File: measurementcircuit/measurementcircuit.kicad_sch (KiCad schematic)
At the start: 17 parts, among them J1 Conn_01x05_Socket, J2 Conn_01x05_Socket

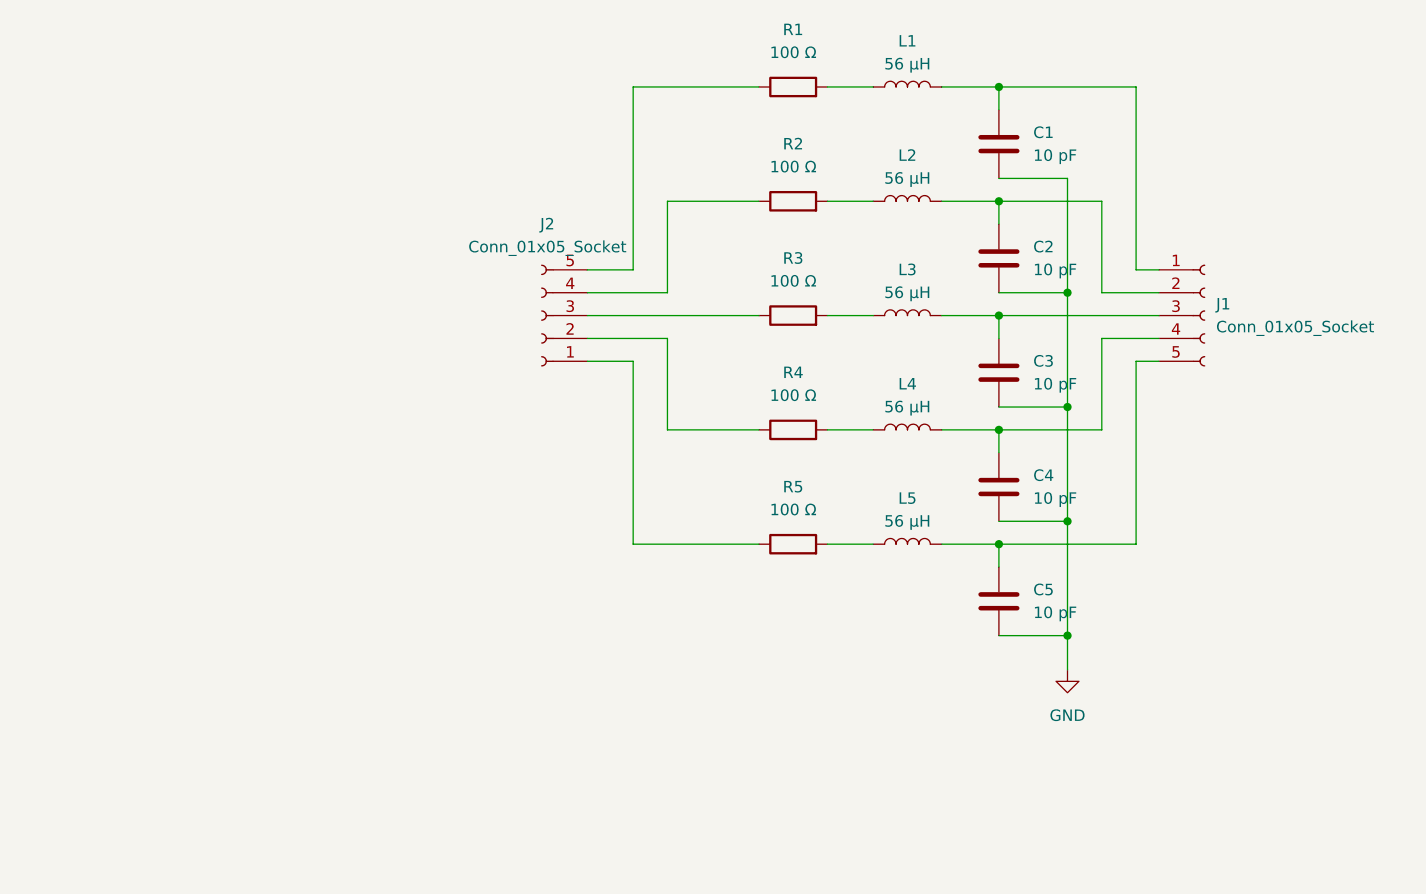
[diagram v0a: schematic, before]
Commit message: Only missing POT
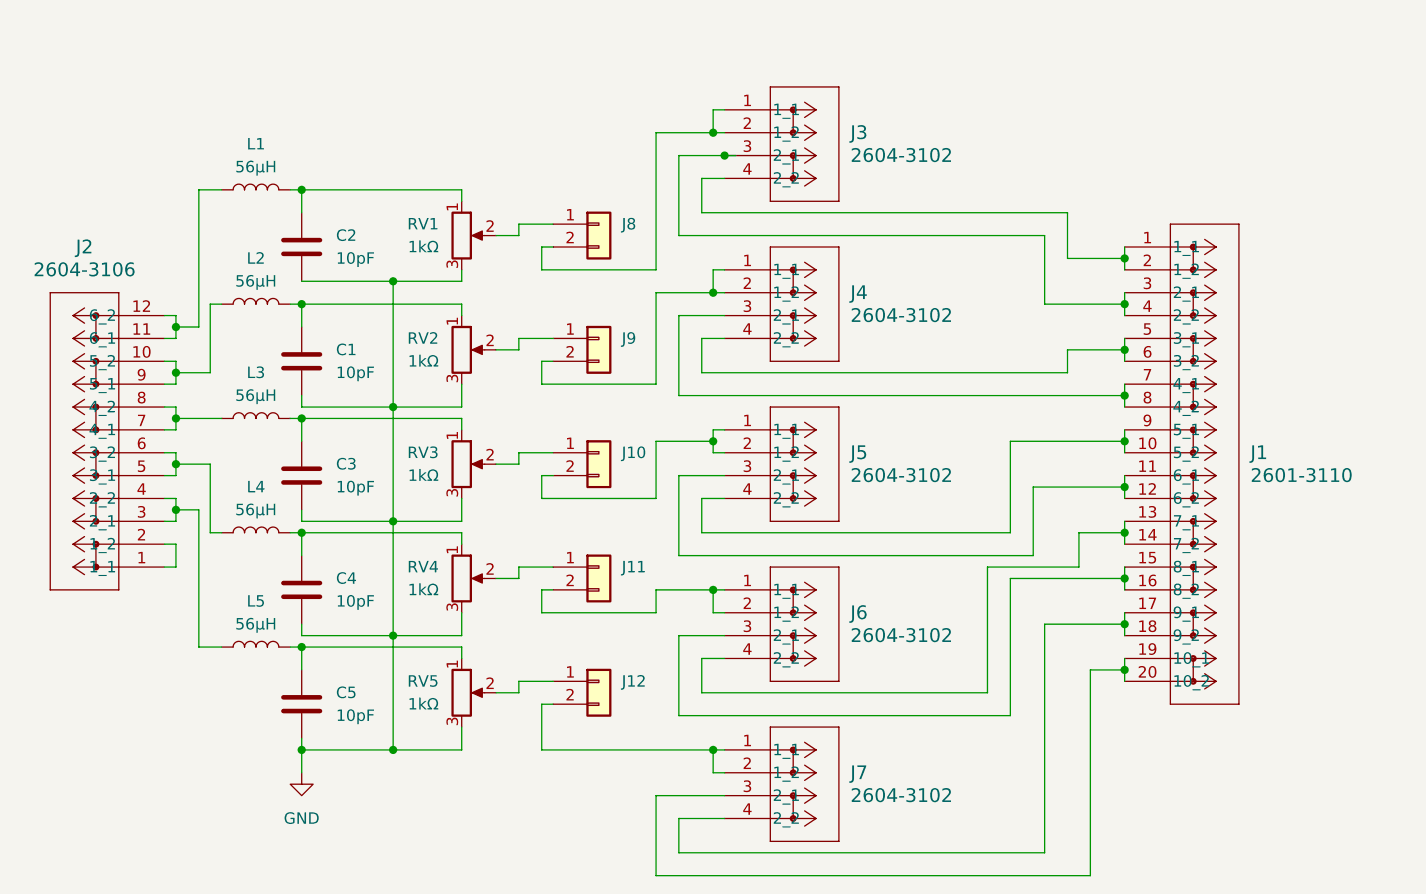
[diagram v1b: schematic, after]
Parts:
- removed J1, J2: Conn_01x05_Socket, Connector_Pin:Pin_D1.3mm_L10.0mm_W3.5mm_Flat, symbol Connector:Conn_01x05_Socket
- removed R1, R2, R3, R4, R5: 100 Ω, Resistor_THT:R_Axial_DIN0204_L3.6mm_D1.6mm_P5.08mm_Horizontal, symbol Device:R
- added J1: 2601-3110, Senior_Design:CONN10_2601-3110_WAG, symbol CONN10:2601-3110
- added J10, J11, J12, J8, J9: Conn_01x02, Connector_PinHeader_2.54mm:PinHeader_1x02_P2.54mm_Vertical, symbol Connector_Generic:Conn_01x02
- added J2: 2604-3106, Senior_Design:CONN6_2604-3106_WAG, symbol CONN6:2604-3106
- added J3, J4, J5, J6, J7: 2604-3102, Senior_Design:CONN2_2604-3102_WAG, symbol CONN2:2604-3102
- added RV1, RV2, RV3, RV4, RV5: 1kΩ, Potentiometer_THT:Potentiometer_ACP_CA9-V10_Vertical, symbol Device:R_Potentiometer
- C1, C2, C3, C4, C5: value 10 pF -> 10pF; footprint Capacitor_THT:CP_Axial_L10.0mm_D4.5mm_P15.00mm_Horizontal -> Capacitor_SMD:C_0805_2012Metric
- L1, L2, L3, L4, L5: value 56 μH -> 56μH; footprint Inductor_THT:L_Axial_L5.0mm_D3.6mm_P10.00mm_Horizontal_Murata_BL01RN1A2A2 -> Inductor_SMD:L_0805_2012Metric
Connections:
- net GND: now also RV1.3, RV2.3, RV3.3, RV4.3, RV5.3
- net at L1.1: now also J2.11 (6_1), J2.12 (6_2)
- net at C2.1: now also L1.2, RV1.1; no longer L2.2
- net at L3.1: now also J2.7 (4_1), J2.8 (4_2)
- net at C1.1: now also L2.2, RV2.1; no longer L1.2
- net at C3.1, L3.2: now also RV3.1
- net at C4.1, L4.2: now also RV4.1
- net at C5.1, L5.2: now also RV5.1
- net at L4.1: now also J2.5 (3_1), J2.6 (3_2)
- net at L5.1: now also J2.3 (2_1), J2.4 (2_2)
- net at L2.1: now also J2.10 (5_2), J2.9 (5_1)
- new net: J9.1 (Pin_1), RV2.2
- new net: J4.1 (1_1), J4.2 (1_2), J9.2 (Pin_2)
- new net: J8.1 (Pin_1), RV1.2
- new net: J10.1 (Pin_1), RV3.2
- new net: J11.1 (Pin_1), RV4.2
- new net: J11.2 (Pin_2), J6.1 (1_1), J6.2 (1_2)
- new net: J1.1 (1_1), J1.2 (1_2), J3.4 (2_2)
- new net: J1.10 (5_2), J1.9 (5_1), J5.4 (2_2)
- new net: J1.11 (6_1), J1.12 (6_2), J5.3 (2_1)
- new net: J1.13 (7_1), J1.14 (7_2), J6.4 (2_2)
- new net: J1.15 (8_1), J1.16 (8_2), J6.3 (2_1)
- new net: J1.17 (9_1), J1.18 (9_2), J7.4 (2_2)
- new net: J1.19 (10_1), J1.20 (10_2), J7.3 (2_1)
- new net: J1.3 (2_1), J1.4 (2_2), J3.3 (2_1)
- new net: J1.5 (3_1), J1.6 (3_2), J4.4 (2_2)
- new net: J1.7 (4_1), J1.8 (4_2), J4.3 (2_1)
- new net: J12.2 (Pin_2), J7.1 (1_1), J7.2 (1_2)
- new net: J2.1 (1_1), J2.2 (1_2)
- new net: J12.1 (Pin_1), RV5.2
- new net: J10.2 (Pin_2), J5.1 (1_1), J5.2 (1_2)
- new net: J3.1 (1_1), J3.2 (1_2), J8.2 (Pin_2)
